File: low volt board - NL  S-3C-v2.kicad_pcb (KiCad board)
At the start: 2 copper layers, 152.4 x 78.7 mm, 42 parts, among them J1 ESP32-S3-ETH-WAVETREE-Footpri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, J2 ILI9341 TFT 2.8" Display with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, J3 4 Channel 5v Relay Connector, J4 SPDT (on)-off-(on), J5 ADC Inputs - 24v side, J6 Dry Contact OptoCoupler, J8 5vIn, Q1-Buzzer1 S8050, SW1 SW_SPDT, U1 ADS1115IDGS - low volt, U2 ADS1115IDGS - 24v, U3-Opto1 PC817

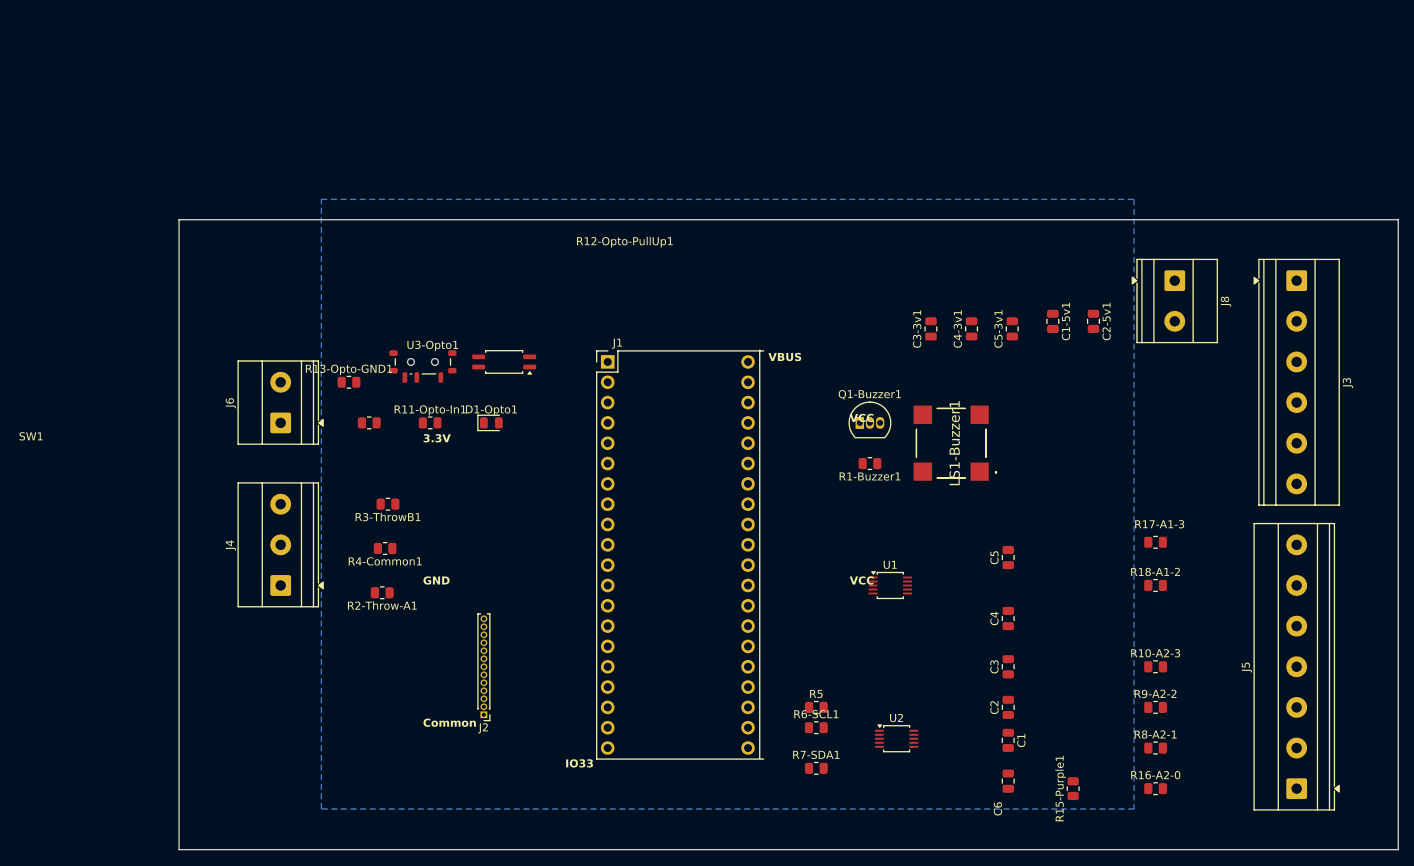
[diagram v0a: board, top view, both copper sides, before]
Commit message: Final design before first autoroute
Co-Authored-By: Claude Opus 4.6 <noreply@anthropic.com>
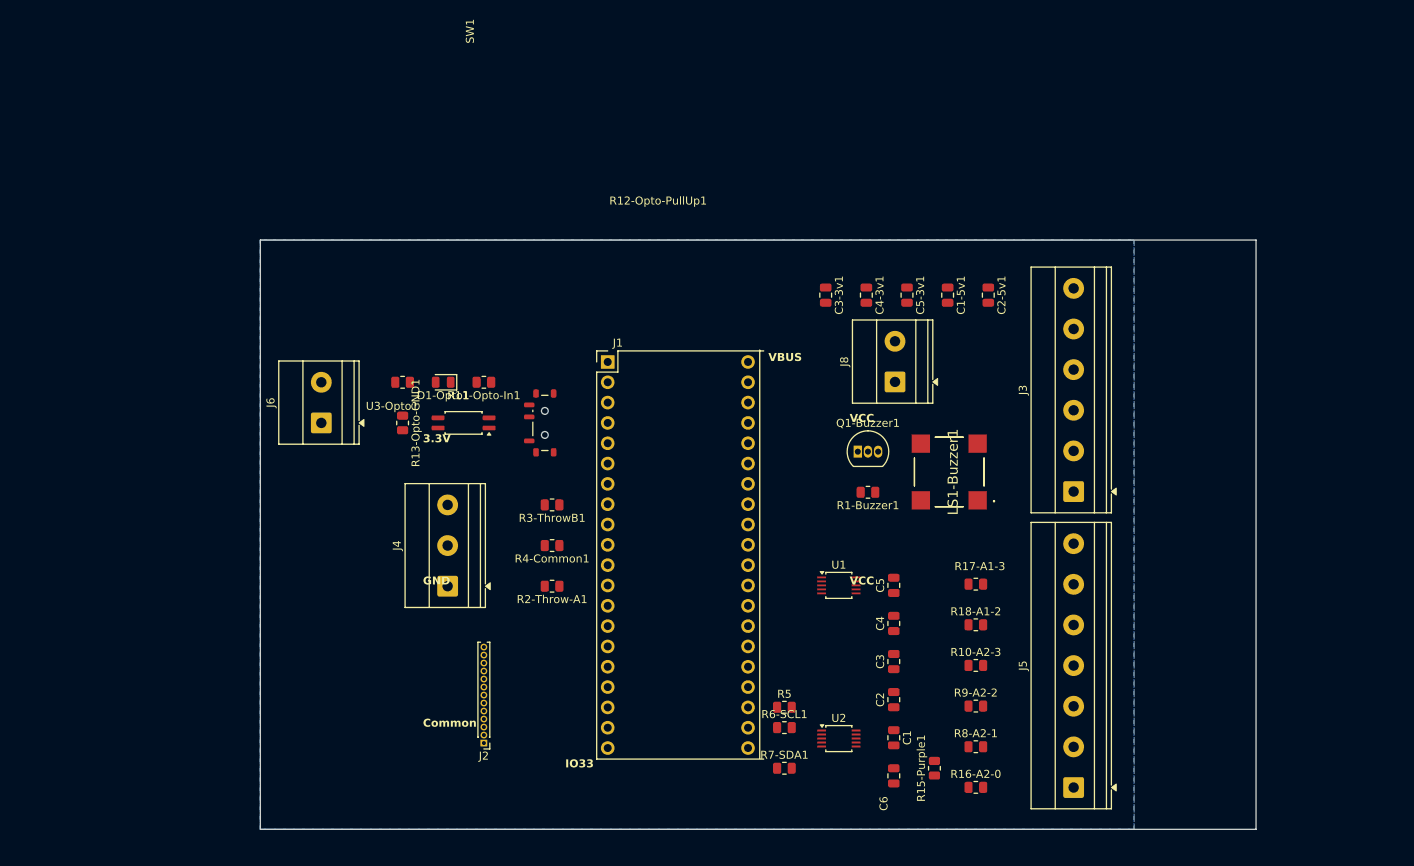
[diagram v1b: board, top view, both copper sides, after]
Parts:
- moved J3 38.4 mm to (155.0, 67.0), turned to 90 degrees
- moved J8 37.2 mm to (132.7, 53.3), turned to 90 degrees
- moved J5 27.9 mm to (155.0, 104.0)
- moved R17-A1-3 23.1 mm to (142.8, 78.6)
- moved R18-A1-2 23.0 mm to (142.8, 83.7)
- moved R10-A2-3 22.5 mm to (142.8, 88.7)
- moved R16-A2-0 22.5 mm to (142.8, 104.0)
- moved R8-A2-1 22.5 mm to (142.8, 98.9)
- moved R9-A2-2 22.5 mm to (142.8, 93.8)
- moved R2-Throw-A1 21.2 mm to (89.8, 78.8)
- moved R4-Common1 20.9 mm to (89.8, 73.8)
- moved J4 20.9 mm to (76.8, 78.8)
- moved R3-ThrowB1 20.5 mm to (89.8, 68.7)
- moved R15-Purple1 17.5 mm to (137.6, 101.6)
- moved SW1 17.0 mm to (88.9, 58.4), turned to 90 degrees
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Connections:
- net /IO21 renamed /Buzer-IO21
- net Net-(LS1-Buzzer1--LEAD) renamed /Buzzer-3
- net Net-(Q1-Buzzer1-B) renamed /Buzzer-2
- J3 pad 1: +5V -> /IO3
- J3 pad 2: GND -> /IO15
- J3 pad 3: /IO16 -> /IO18
- J3 pad 4: /IO18 -> /IO16
- J3 pad 5: /IO15 -> GND
- J3 pad 6: /IO3 -> +5V
- J5 pad 6: /A1-2-E -> /A1-3-E
- J8 pad 1: +5V -> GND
- J8 pad 2: GND -> +5V
- R8-A2-1 pad 1: /A2-1 -> /A2-1-E
- R8-A2-1 pad 2: /A2-1-E -> /A2-1
- R9-A2-2 pad 1: /A2-2 -> /A2-2-E
- R9-A2-2 pad 2: /A2-2-E -> /A2-2
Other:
- board size 152.4 x 78.7 mm -> 124.5 x 73.7 mm
